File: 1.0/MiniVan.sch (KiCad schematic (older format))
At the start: 246 parts, among them J1 Reset Switch - A, J2 Reset Switch - B, J3 Reset Switch - C, U1 Elite-C - A, U2 Elite-C - B, U3 Elite-C - C

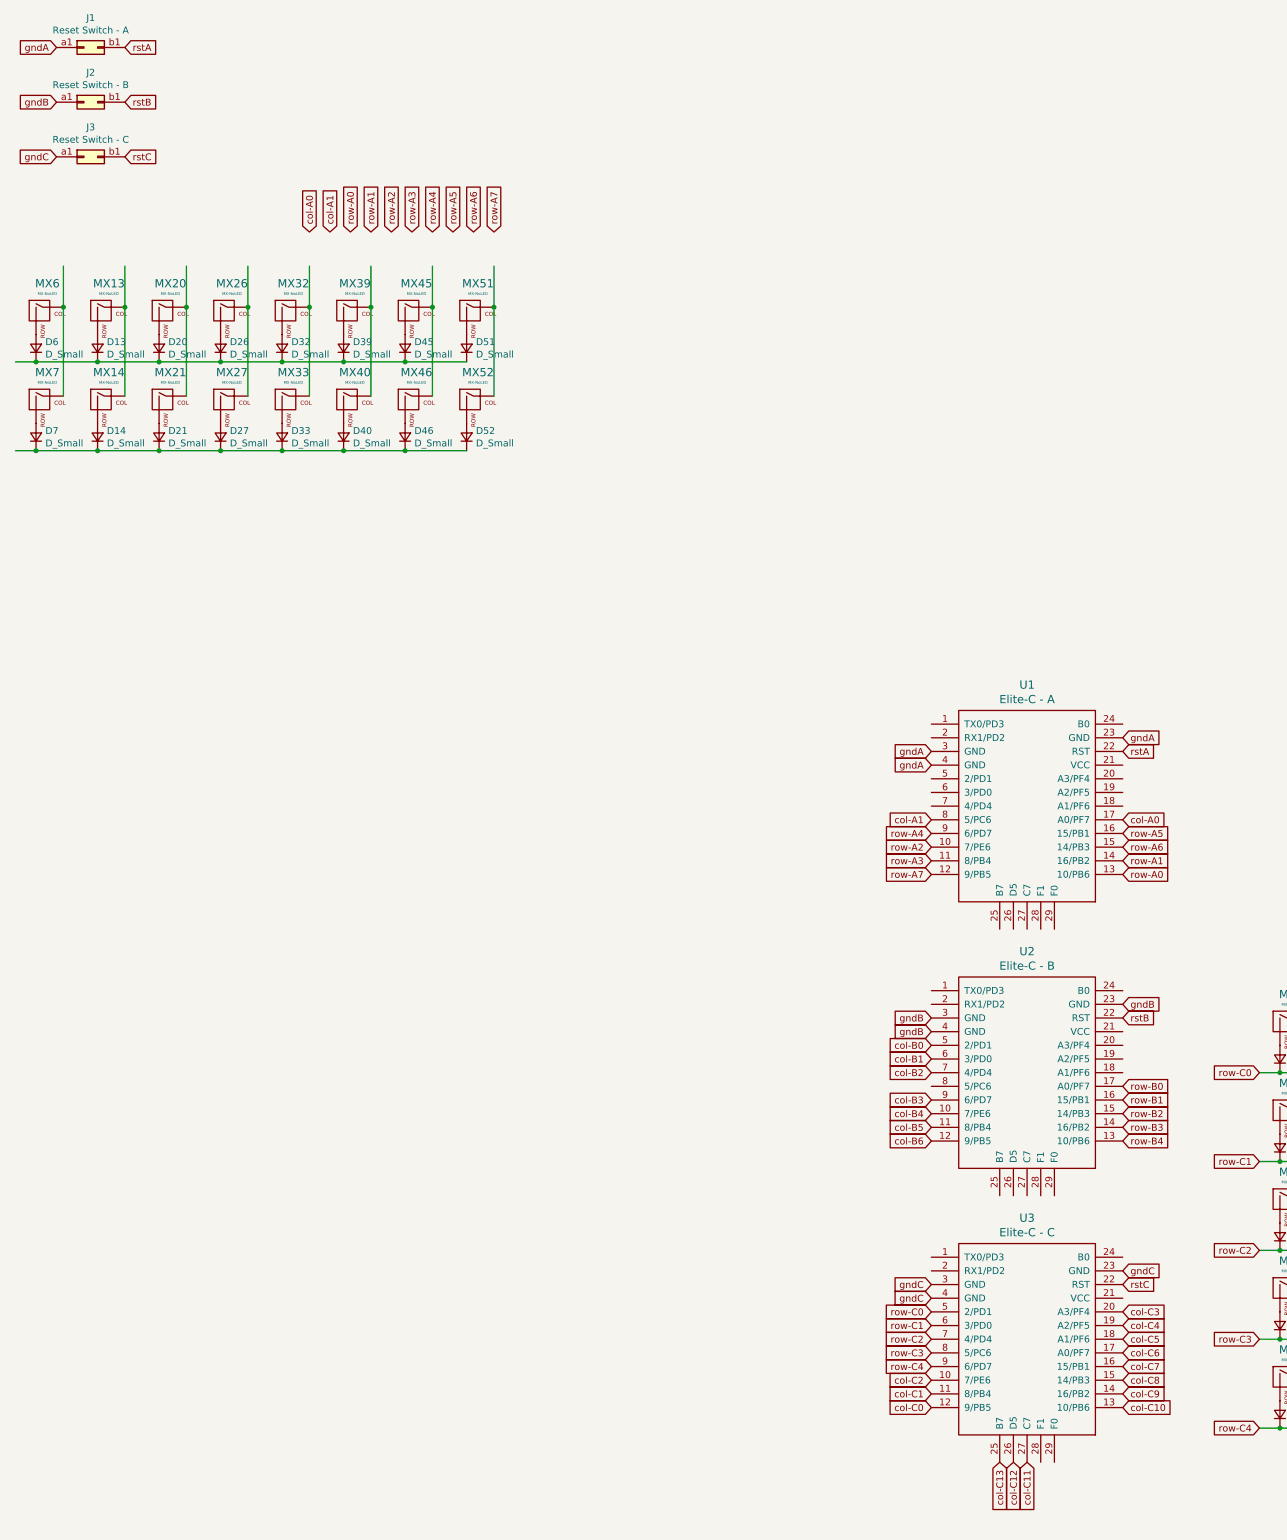
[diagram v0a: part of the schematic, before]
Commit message: 4/30/20 v1
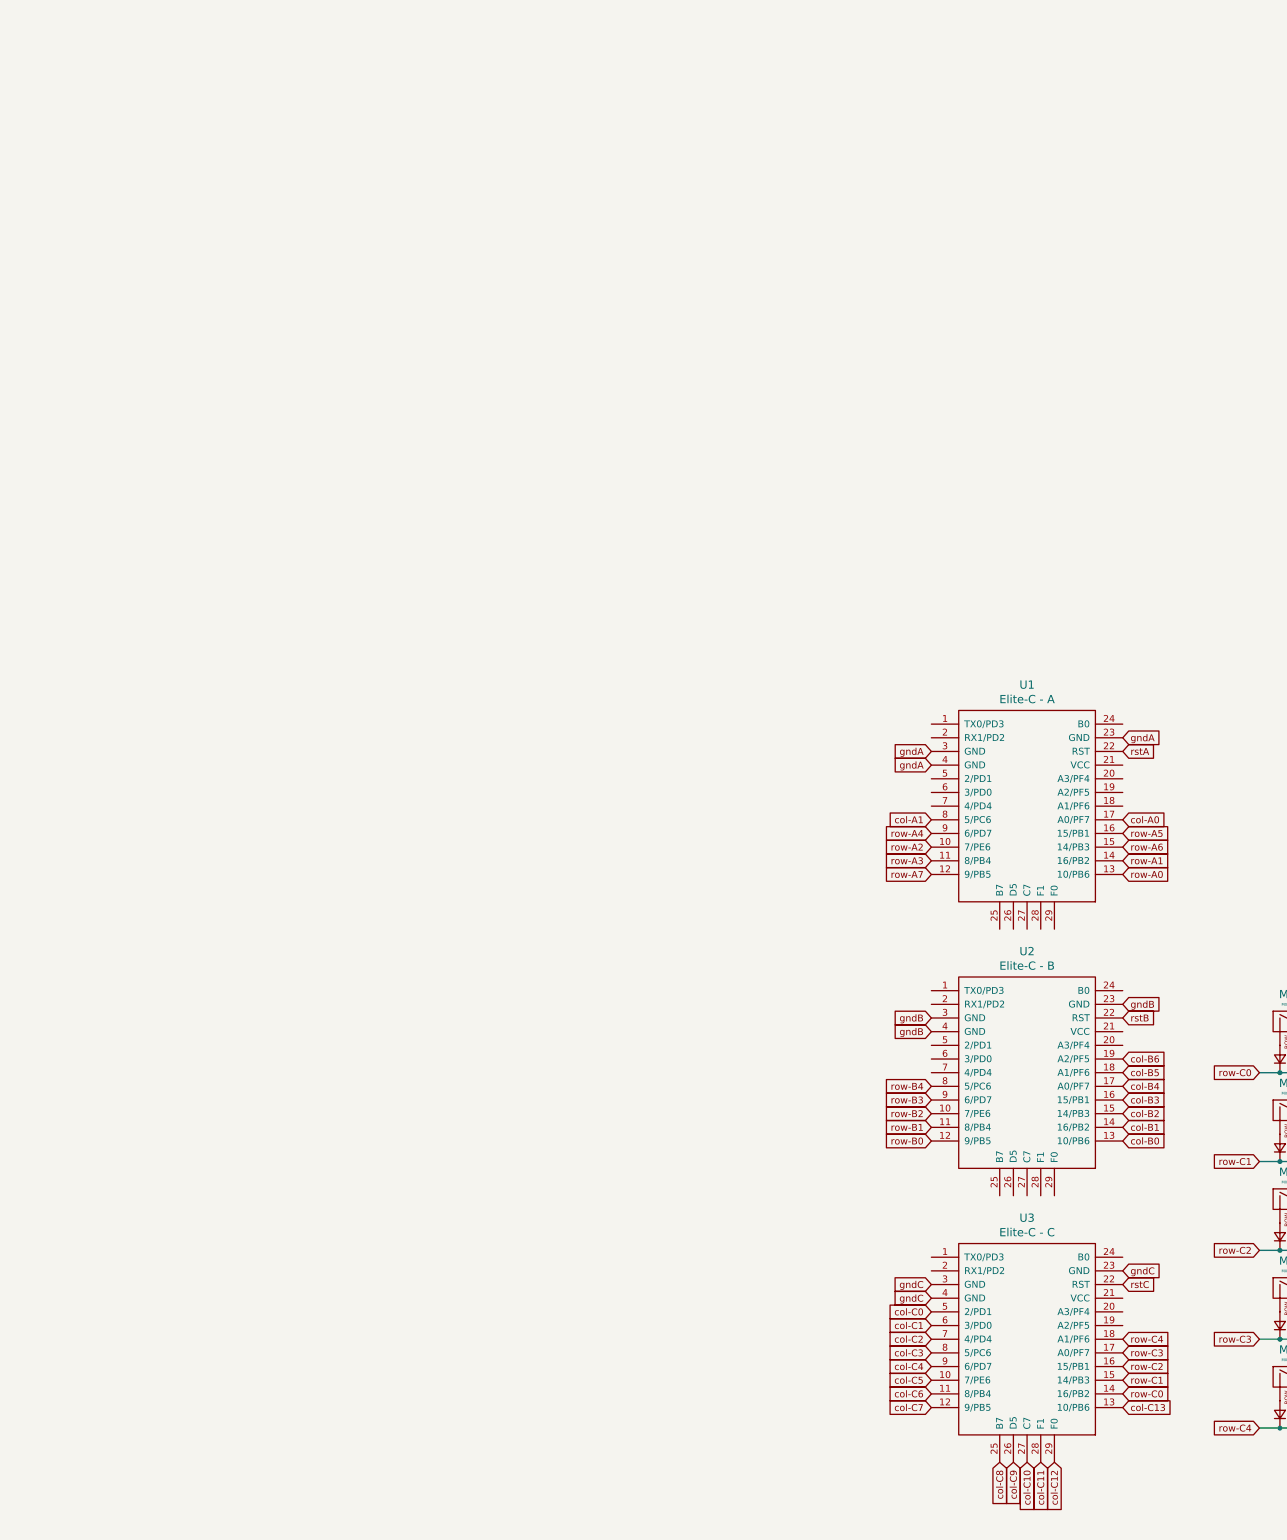
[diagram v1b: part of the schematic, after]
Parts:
- removed D13, D14, D20, D21, D26, D27, D32, D33, D39, D40, D45, D46, D51, D52, D6, D7: D_Small, Diode_THT:D_DO-35_SOD27_P3.81mm_Vertical_AnodeUp, symbol Device:D_Small
- removed J1: Reset Switch - A, Connector_Wire:SolderWirePad_1x02_P3.81mm_Drill0.8mm, symbol Connector_Generic:Conn_02x01_Row_Letter_First
- removed J2: Reset Switch - B, Connector_Wire:SolderWirePad_1x02_P3.81mm_Drill0.8mm, symbol Connector_Generic:Conn_02x01_Row_Letter_First
- removed J3: Reset Switch - C, Connector_Wire:SolderWirePad_1x02_P3.81mm_Drill0.8mm, symbol Connector_Generic:Conn_02x01_Row_Letter_First
- removed MX13, MX14, MX20, MX21, MX26, MX27, MX32, MX33, MX39, MX40, MX45, MX46, MX51, MX52, MX6, MX7: MX-NoLED, MX_Alps_Hybrid:MX-1U-NoLED, symbol MX_Alps_Hybrid:MX-NoLED
- MX4: footprint MX_Alps_Hybrid:MX-2U-NoLED -> MX_Alps_Hybrid:MX-2.25U-NoLED
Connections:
- wire segments 241 -> 209

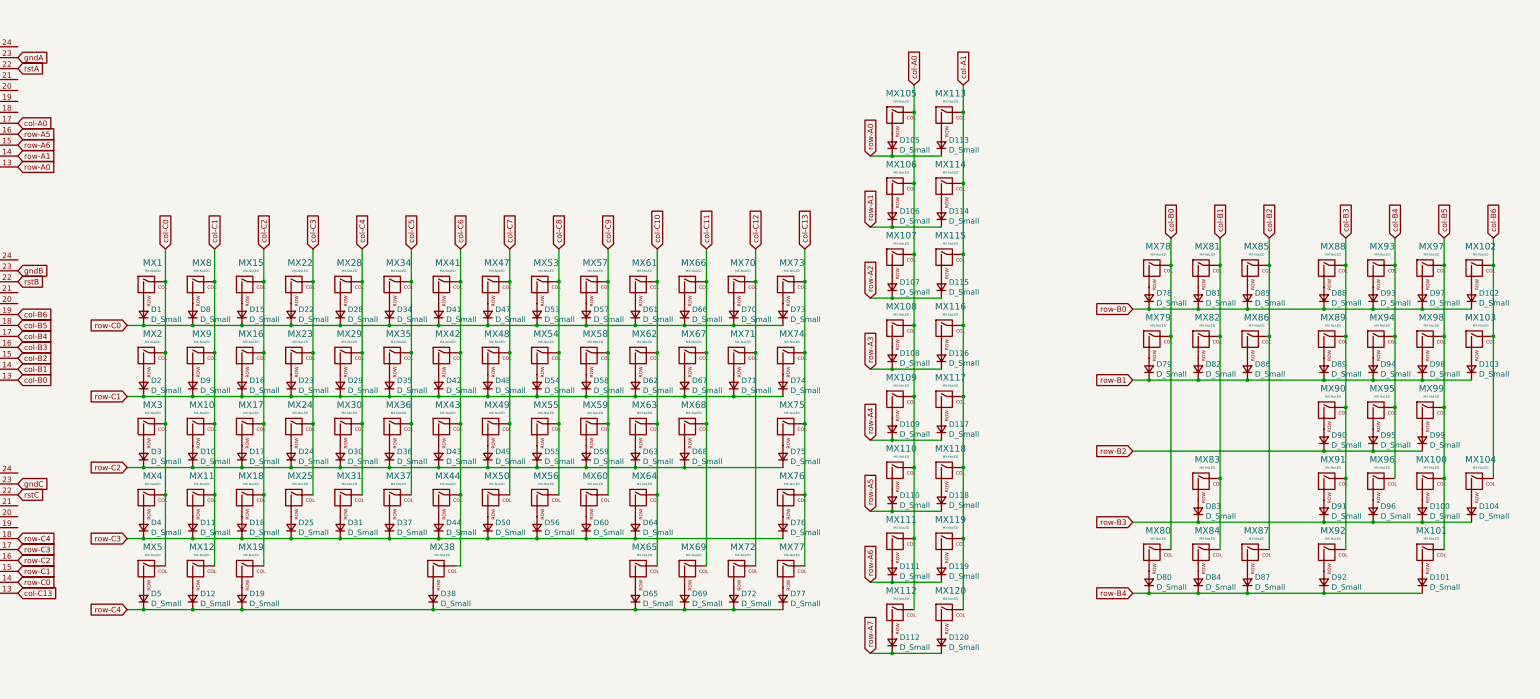
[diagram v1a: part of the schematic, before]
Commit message: 5/1/20 v1
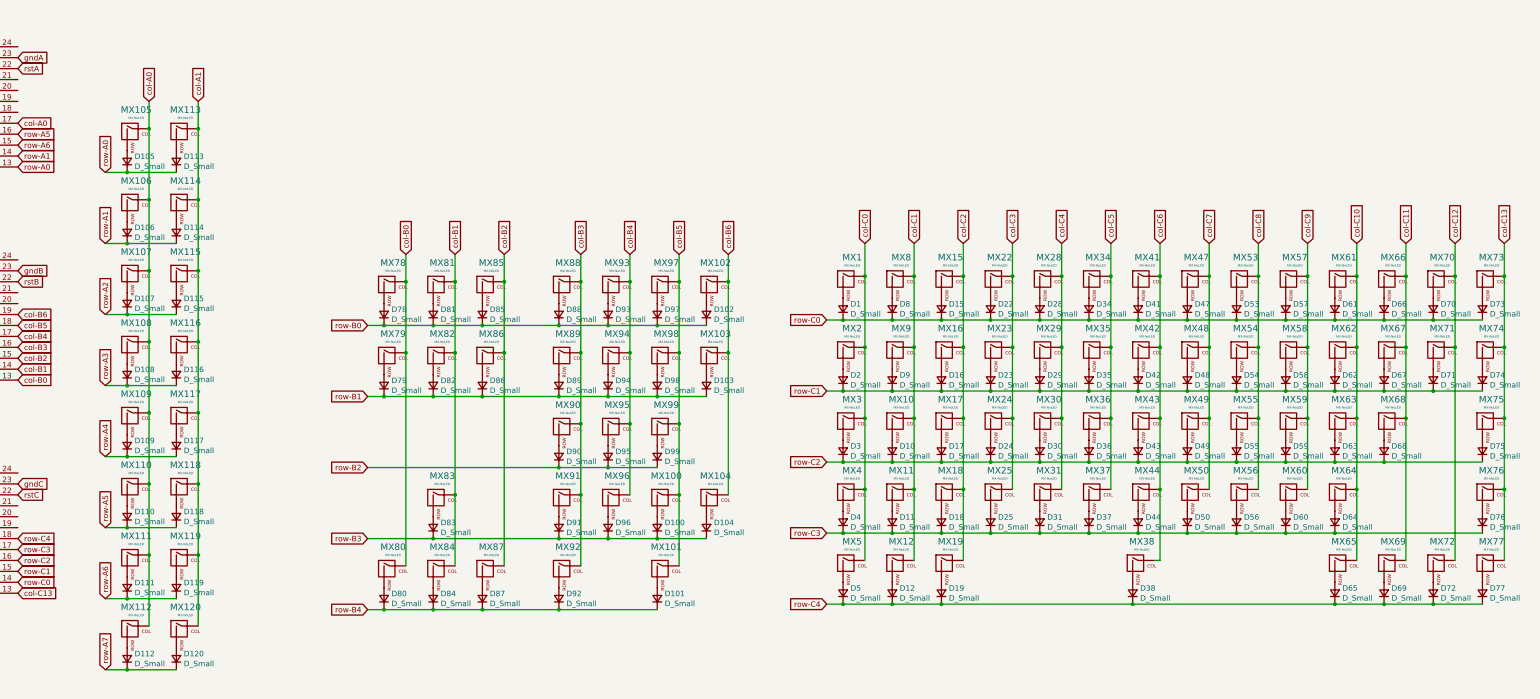
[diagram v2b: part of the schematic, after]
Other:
- moved on the sheet: D1, D10, D100, D101, D102, D103, D104, D105, D106, D107, D108, D109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
